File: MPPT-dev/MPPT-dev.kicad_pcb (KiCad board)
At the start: 2 copper layers, 50 x 50 mm, 29 parts, among them J1 200528-0100, J13 282834-6, J2 Conn_01x02, Q1 PMOS, U1 LTC4412xS6, U2 LT8611EUDD-PBF, U3 AD5245BRJZ10-R2

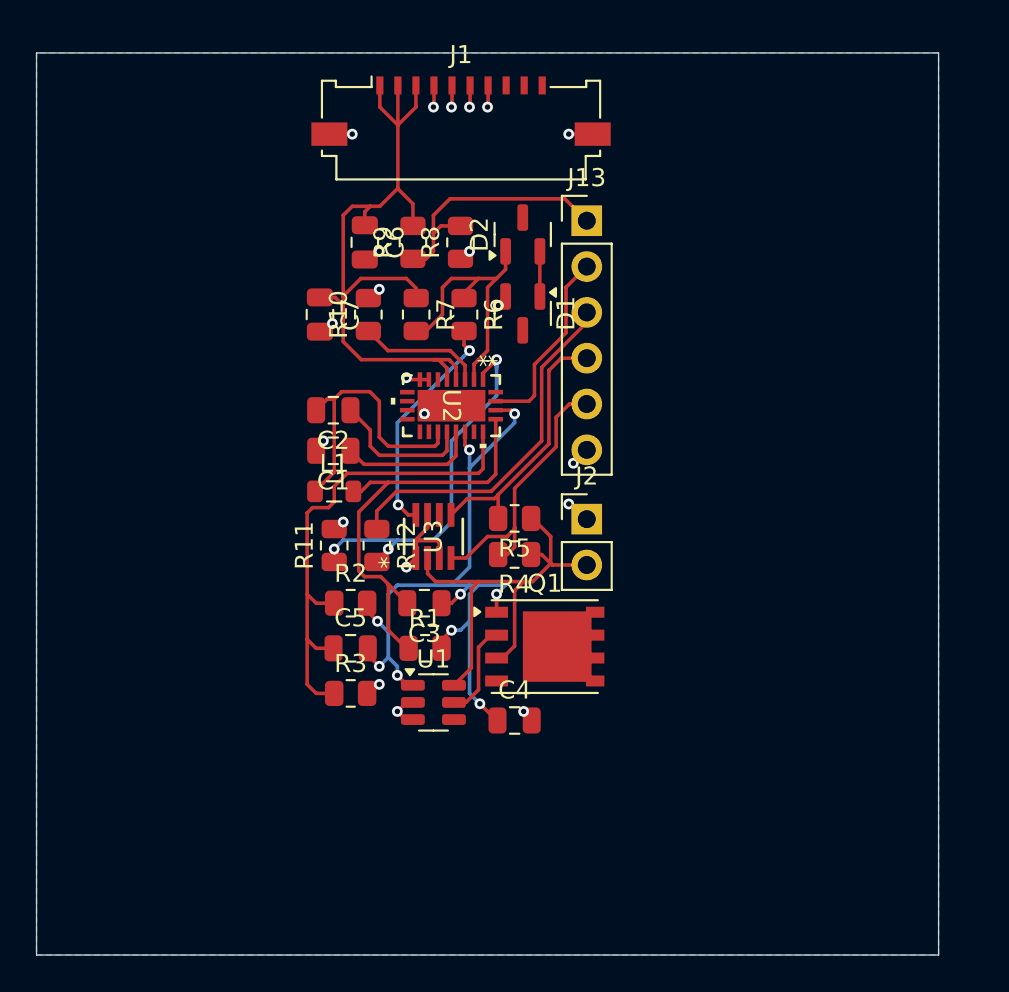
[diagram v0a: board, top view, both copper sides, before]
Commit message: Board review
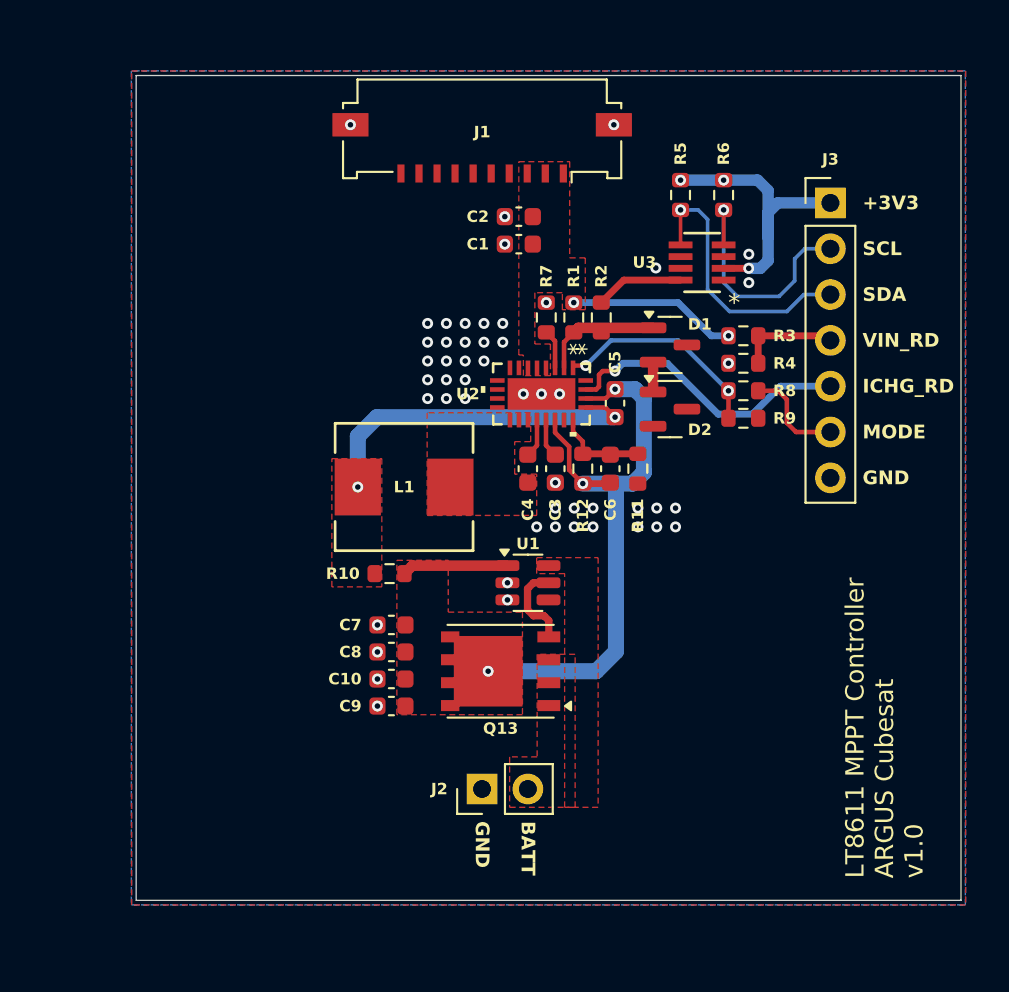
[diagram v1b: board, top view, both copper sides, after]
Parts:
- removed J13: 282834-6, Connector_PinHeader_2.54mm:PinHeader_1x06_P2.54mm_Vertical
- removed Q1: PMOS, Package_SO:PowerPAK_SO-8_Single
- added C10: 10u, Capacitor_SMD:C_0603_1608Metric, F.Cu at (134.7, 109.7)
- added C8: 10u, Capacitor_SMD:C_0603_1608Metric, F.Cu at (134.7, 108.2)
- added C9: 10u, Capacitor_SMD:C_0603_1608Metric, F.Cu at (134.7, 111.2)
- added J3: Conn_01x07, Connector_PinHeader_2.54mm:PinHeader_1x07_P2.54mm_Vertical, F.Cu at (159.0, 83.3)
- added Q13: SIRA99DP-T1-GE3, Package_SO:PowerPAK_SO-8_Single, F.Cu at (140.7, 109.3)
- C1: value 1u -> 22u; footprint Capacitor_SMD:C_0805_2012Metric -> Capacitor_SMD:C_0603_1608Metric
- C2: value 0.1u -> 4u7; footprint Capacitor_SMD:C_0805_2012Metric -> Capacitor_SMD:C_0603_1608Metric
- C3: footprint Capacitor_SMD:C_0805_2012Metric -> Capacitor_SMD:C_0603_1608Metric
- C4: value 0.1u -> 100n; footprint Capacitor_SMD:C_0805_2012Metric -> Capacitor_SMD:C_0603_1608Metric
- C5: value 10p -> 1u; footprint Capacitor_SMD:C_0805_2012Metric -> Capacitor_SMD:C_0603_1608Metric
- C6: value 4.7u -> 10p; footprint Capacitor_SMD:C_0805_2012Metric -> Capacitor_SMD:C_0603_1608Metric
- C7: value 22u -> 10u; footprint Capacitor_SMD:C_0805_2012Metric -> Capacitor_SMD:C_0603_1608Metric
- J1: footprint Argus-Connectors:Molex_200528-0100_1x10-1MP_P1.00mm_Horizontal -> footprints:Molex_200528-0100_1x10-1MP_P1.00mm_Horizontal
- L1: value 4.7u -> 4u7; footprint Inductor_SMD:L_0805_2012Metric -> footprints:IND_03-4R7-R_EAT
- R1: value 50m -> 309k; footprint Resistor_SMD:R_0805_2012Metric -> Resistor_SMD:R_0603_1608Metric
- R10: value 60.4K -> 50m; footprint Resistor_SMD:R_0805_2012Metric -> Resistor_SMD:R_0603_1608Metric
- R11: value 0 -> 130k; footprint Resistor_SMD:R_0805_2012Metric -> Resistor_SMD:R_0603_1608Metric
- R12: value 0 -> 1M; footprint Resistor_SMD:R_0805_2012Metric -> Resistor_SMD:R_0603_1608Metric
- R2: value 1M -> 6k2; footprint Resistor_SMD:R_0805_2012Metric -> Resistor_SMD:R_0603_1608Metric
- R3: value 309K -> ?R; footprint Resistor_SMD:R_0805_2012Metric -> Resistor_SMD:R_0603_1608Metric
- R4: value 10K -> ?R; footprint Resistor_SMD:R_0805_2012Metric -> Resistor_SMD:R_0603_1608Metric
- R5: value 10K -> 10k; footprint Resistor_SMD:R_0805_2012Metric -> Resistor_SMD:R_0603_1608Metric
- R6: value 6.2K -> 10k; footprint Resistor_SMD:R_0805_2012Metric -> Resistor_SMD:R_0603_1608Metric
- R7: value 309K -> 60k4; footprint Resistor_SMD:R_0805_2012Metric -> Resistor_SMD:R_0603_1608Metric
- R8, R9: value R_Small -> 0R; footprint Resistor_SMD:R_0805_2012Metric -> Resistor_SMD:R_0603_1608Metric
- moved R3 29.4 mm to (154.2, 90.7), turned to 180 degrees
- moved U3 21.3 mm to (151.9, 86.6), turned to 180 degrees
- moved R2 21.1 mm to (146.3, 89.7), turned to 90 degrees
- moved R9 20.7 mm to (154.2, 95.2), turned to 0 degrees
- moved R5 20.1 mm to (150.7, 82.9), turned to -90 degrees
- moved R1 20.1 mm to (144.8, 89.7), turned to -90 degrees
- moved C5 20.0 mm to (147.1, 94.4), turned to -90 degrees
- moved C6 18.5 mm to (146.8, 98.0)
- moved R8 17.7 mm to (154.2, 93.7), turned to 180 degrees
- moved C7 17.7 mm to (134.7, 106.7), turned to 180 degrees
- moved R11 17.4 mm to (148.3, 98.0), turned to -90 degrees
- moved R4 16.5 mm to (154.2, 92.2), turned to 0 degrees
- moved J2 16.0 mm to (139.7, 115.8), turned to 90 degrees
- moved R6 15.8 mm to (153.1, 82.9)
- moved C1 15.4 mm to (141.7, 85.6)
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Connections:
- C1 pad 1: /MPPT/INTVcc -> /D_VSOLAR1
- C2 pad 1: /MPPT/BST -> /D_VSOLAR1
- C2 pad 2: /MPPT/SW1 -> GND
- C3 pad 1: /MPPT/BIAS -> /MPPT/INTVcc
- C3 pad 2: /MPPT/ISP -> GND
- C4 pad 1: /MPPT/BIAS -> /MPPT/BST
- C4 pad 2: GND -> /MPPT/SW
- C5 pad 1: /MPPT/FB -> /MPPT/BIAS
- C5 pad 2: /MPPT/BIAS -> /MPPT/ISP
- C6 pad 1: D_VSOLAR1 -> /MPPT/FB
- C6 pad 2: GND -> /MPPT/BIAS
- C7 pad 1: D_VSOLAR1 -> /MPPT/BIAS
- D1 pad 1: Net-(D2-A) -> /MPPT/MP_CTRL
- D1 pad 2: GND -> Net-(D1-A)
- D2 pad 1: /MPPT/MP_CTRL -> Net-(D1-A)
- D2 pad 2: Net-(D2-A) -> GND
- J1 pad 1: D_VSOLAR1 -> /D_VSOLAR1
- J1 pad 2: D_VSOLAR1 -> /D_VSOLAR1
- J1 pad 3: D_VSOLAR1 -> /D_VSOLAR1
- L1 pad 1: /MPPT/SW1 -> /MPPT/SW
- R1 pad 1: /MPPT/ISP -> /D_VSOLAR1
- R1 pad 2: /MPPT/BIAS -> /MPPT/MP_CTRL
- R10 pad 1: /MPPT/RT -> /MPPT/ISP
- R10 pad 2: GND -> /MPPT/BIAS
- R11 pad 1: /MPPT/SYNC -> /MPPT/FB
- R12 pad 1: /MODE -> /MPPT/FB
- R12 pad 2: /MPPT/SYNC -> /MPPT/BIAS
- R2 pad 1: /MPPT/FB -> /MPPT/MP_CTRL
- R2 pad 2: /MPPT/BIAS -> /MPPT/A
- R3 pad 1: /MPPT/FB -> /VIN_RD
- R3 pad 2: GND -> /D_VSOLAR1
- R4 pad 1: /BATTERY -> GND
- R4 pad 2: /SCL -> /VIN_RD
- R5 pad 1: /BATTERY -> +3V3
- R6 pad 1: /MPPT/MP_CTRL -> +3V3
- R6 pad 2: /MPPT/A -> /SCL
- R7 pad 1: D_VSOLAR1 -> /MPPT/RT
- R7 pad 2: /MPPT/MP_CTRL -> GND
- R8 pad 1: GND -> /MODE
- R8 pad 2: /VIN_RD -> /MPPT/SYNC
- R9 pad 1: /VIN_RD -> /MPPT/SYNC
- R9 pad 2: D_VSOLAR1 -> GND
- U2 pad 10: unconnected-(U2-NC-Pad10) -> GND
- U2 pad 11: unconnected-(U2-NC-Pad11) -> GND
- U2 pad 12: unconnected-(U2-NC-Pad12) -> GND
- U2 pad 13: unconnected-(U2-SW-Pad13) -> /MPPT/SW
- U2 pad 14: unconnected-(U2-SW-Pad14) -> /MPPT/SW
- U2 pad 15: /MPPT/SW1 -> /MPPT/SW
- U2 pad 4: D_VSOLAR1 -> /D_VSOLAR1
- U2 pad 5: D_VSOLAR1 -> /D_VSOLAR1
- U2 pad 6: unconnected-(U2-VIN-Pad6) -> /D_VSOLAR1
- U2 pad 9: unconnected-(U2-NC-Pad9) -> GND
- U3 pad 2: /BATTERY -> +3V3
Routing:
- net D_VSOLAR1: track 41.0 -> 0.00 mm
- net GND: track 27.1 -> 0.00 mm, vias 21 -> 52
- net /BATTERY: track 26.0 -> 0.00 mm
- net /MPPT/FB: track 27.9 -> 5.18 mm
- net +3V3: track 0.00 -> 16.6 mm, vias 0 -> 3
- net /MPPT/SW1: track 15.9 -> 0.00 mm
- net /MODE: track 19.9 -> 5.71 mm
- net /MPPT/SYNC: track 21.5 -> 11.9 mm, vias 3 -> 2
- net /D_VSOLAR1: track 0.00 -> 9.34 mm, vias 0 -> 2
- net /MPPT/MP_CTRL: track 15.8 -> 6.69 mm
- net /VIN_RD: track 14.4 -> 5.63 mm
- net /MPPT/A: track 12.6 -> 4.91 mm, vias 2 -> 0
- net /MPPT/BST: track 8.07 -> 2.13 mm
- net /ICHG_RD: track 10.6 -> 16.4 mm, vias 0 -> 1
- net /MPPT/INTVcc: track 7.69 -> 2.13 mm
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- added copper zone on F.Cu, net /BATTERY
- added copper zone on F.Cu, net /D_VSOLAR1
- added copper zone on F.Cu, net /MPPT/BIAS
- added copper zone on F.Cu, net /MPPT/ISP
- added copper zone on F.Cu, net /MPPT/SW
- added copper zone on F.Cu, net GND
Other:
- board size 50 x 50 mm -> 45.7 x 45.7 mm
- board text added: "+3V3"
- board text added: "BATT"
- board text added: "GND"
- board text added: "ICHG_RD"
- board text added: "LT8611 MPPT Controller ARGUS Cubesat v1.0"
- board text added: "MODE"
- board text added: "SCL"
- board text added: "SDA"
- board text added: "VIN_RD"
